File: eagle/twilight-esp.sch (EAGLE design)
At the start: 12 parts, among them IC1 7805T, J1 Mini PIR, J2 VOUT, J3 VIN, Q1 IRF540

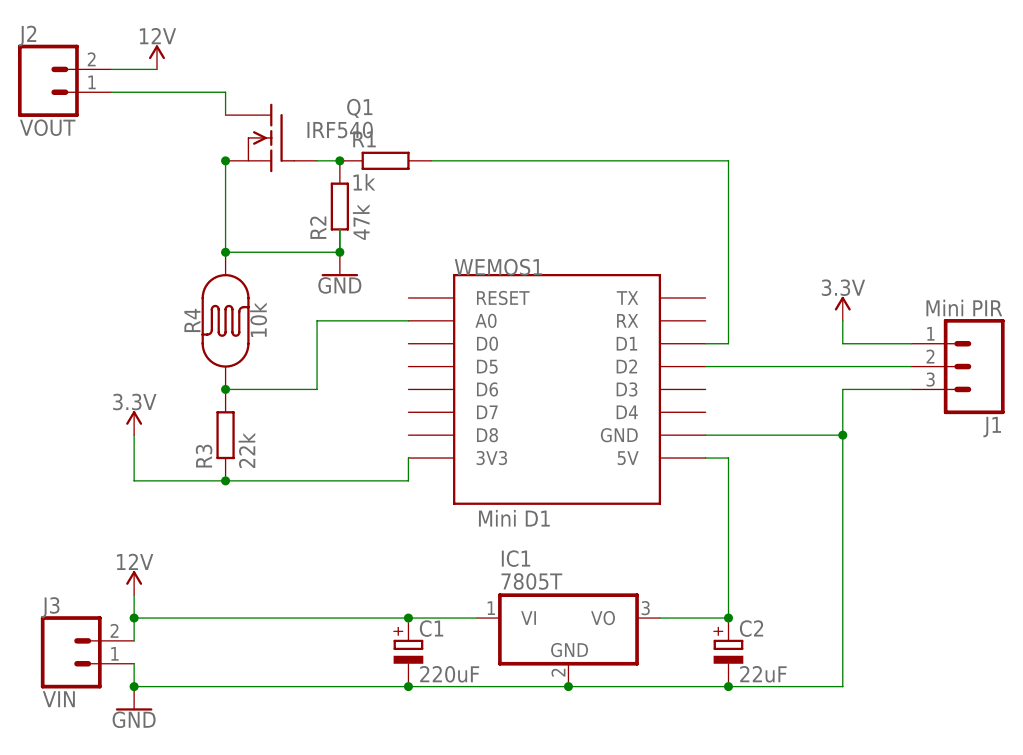
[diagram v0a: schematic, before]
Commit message: add reset header
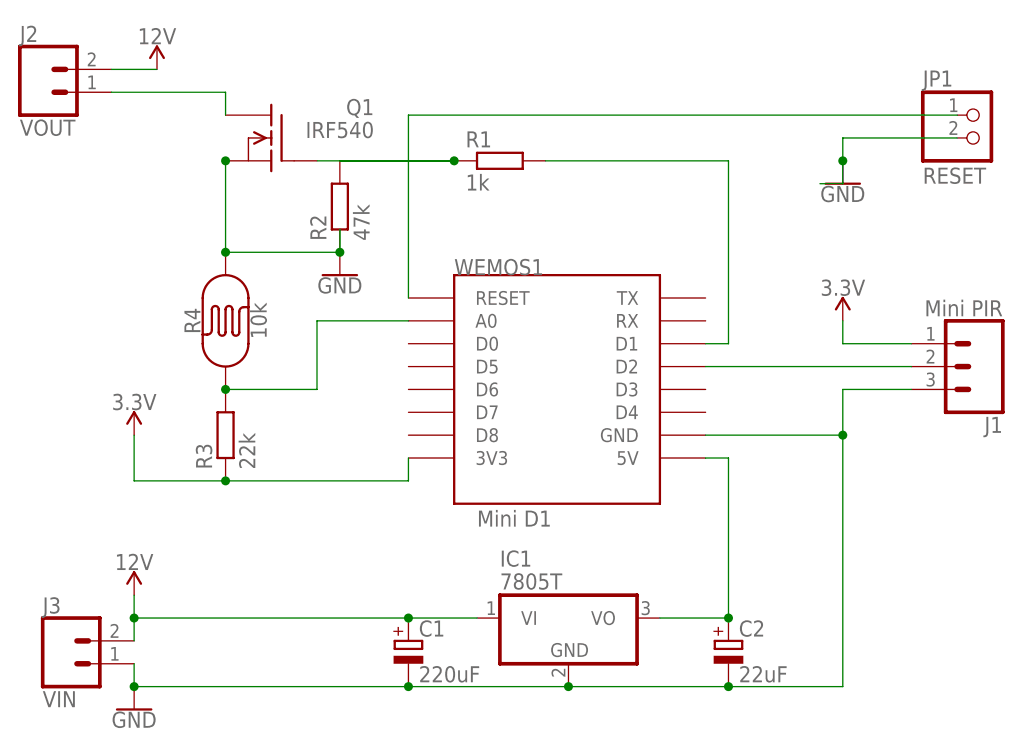
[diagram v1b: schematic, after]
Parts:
- added JP1: RESET, pinhead:PINHD-1X2
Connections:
- new net N$4: JP1.1, WEMOS1.RESET
- net GND: now also JP1.2
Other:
- moved on the sheet: R1
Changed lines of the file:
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@@
 <part name="R2" library="rcl" deviceset="R-EU_" device="0207/7" value="47k"/>
 <part name="R3" library="rcl" deviceset="R-EU_" device="0207/7" value="22k"/>
+<part name="JP1" library="pinhead" deviceset="PINHD-1X2" device="" value="RESET"/>
+<part name="GND2" library="SparkFun-PowerSymbols" deviceset="GND" device=""/>
 </parts>
 <sheets>
@@
 <instance part="IC1" gate="A1" x="45.72" y="43.18"/>
 <instance part="Q1" gate="G$1" x="12.7" y="96.52" rot="MR0"/>
-<instance part="R1" gate="G$1" x="25.4" y="93.98"/>
+<instance part="R1" gate="G$1" x="38.1" y="93.98"/>
 <instance part="R2" gate="G$1" x="20.32" y="88.9" rot="R90"/>
 <instance part="R3" gate="G$1" x="7.62" y="63.5" rot="R90"/>
+<instance part="JP1" gate="G$1" x="91.44" y="96.52"/>
+<instance part="GND2" gate="1" x="76.2" y="91.44"/>
 </instances>
 <busses>
@@
 <junction x="7.62" y="93.98"/>
 <pinref part="R2" gate="G$1" pin="1"/>
+</segment>
+<segment>
+<pinref part="GND2" gate="1" pin="GND"/>
+<wire x1="73.66" y1="91.44" x2="76.2" y2="91.44" width="0.1524" layer="91"/>
+<wire x1="76.2" y1="91.44" x2="76.2" y2="93.98" width="0.1524" layer="91"/>
+<wire x1="76.2" y1="93.98" x2="76.2" y2="96.52" width="0.1524" layer="91"/>
+<pinref part="JP1" gate="G$1" pin="2"/>
+<wire x1="76.2" y1="96.52" x2="88.9" y2="96.52" width="0.1524" layer="91"/>
+<junction x="76.2" y="93.98"/>
 </segment>
 </net>
@@
 <net name="N$1" class="0">
 <segment>
-<wire x1="30.48" y1="93.98" x2="63.5" y2="93.98" width="0.1524" layer="91"/>
+<wire x1="43.18" y1="93.98" x2="63.5" y2="93.98" width="0.1524" layer="91"/>
 <wire x1="63.5" y1="93.98" x2="63.5" y2="73.66" width="0.1524" layer="91"/>
 <pinref part="WEMOS1" gate="D1" pin="D1"/>
@@
 <segment>
 <pinref part="Q1" gate="G$1" pin="G"/>
-<wire x1="17.78" y1="93.98" x2="20.32" y2="93.98" width="0.1524" layer="91"/>
+<wire x1="17.78" y1="93.98" x2="33.02" y2="93.98" width="0.1524" layer="91"/>
 <pinref part="R1" gate="G$1" pin="1"/>
 <pinref part="R2" gate="G$1" pin="2"/>
-<junction x="20.32" y="93.98"/>
+<junction x="33.02" y="93.98"/>
+<wire x1="33.02" y1="93.98" x2="20.32" y2="93.98" width="0.1524" layer="91"/>
 </segment>
 </net>
@@
 </segment>
 </net>
+<net name="N$4" class="0">
+<segment>
+<pinref part="WEMOS1" gate="D1" pin="RESET"/>
+<wire x1="27.94" y1="78.74" x2="27.94" y2="99.06" width="0.1524" layer="91"/>
+<pinref part="JP1" gate="G$1" pin="1"/>
+<wire x1="27.94" y1="99.06" x2="88.9" y2="99.06" width="0.1524" layer="91"/>
+</segment>
+</net>
